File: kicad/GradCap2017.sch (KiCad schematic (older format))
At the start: 14 parts

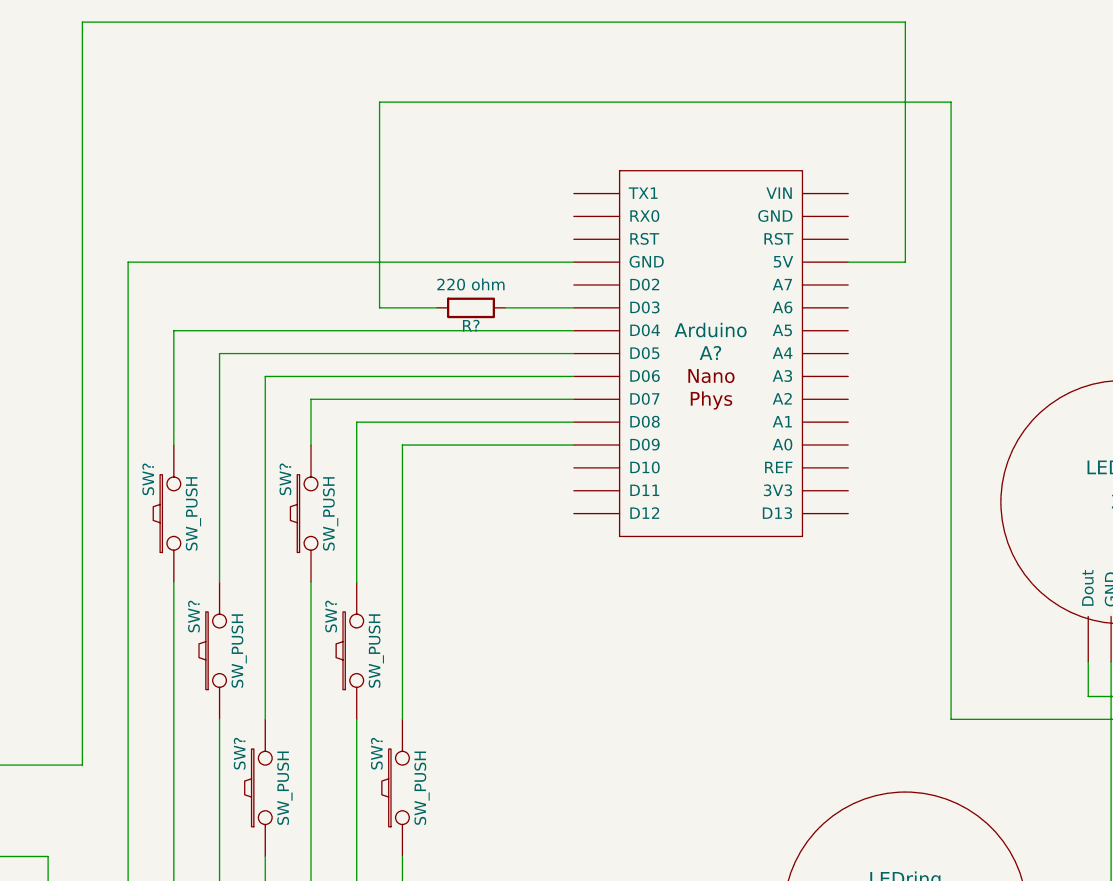
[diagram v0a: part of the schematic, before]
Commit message: add buttons
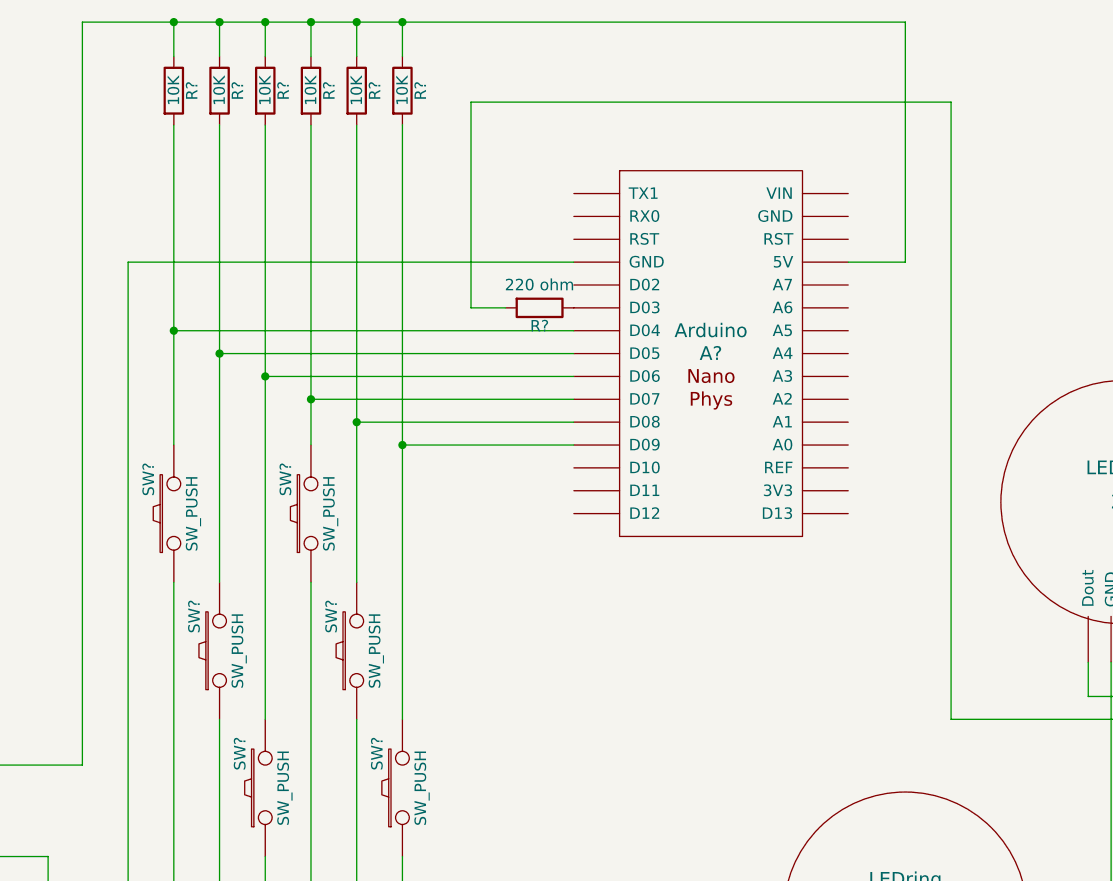
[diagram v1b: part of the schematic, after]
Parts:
- added R? (x6): 10K, symbol R
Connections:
- net at Z?.~ (GND): now also R?.2; no longer Z?.~ (GND)
- net at A?.~ (VIN): now also SW?.2, R?.2; no longer J?.~ (Vout)
- net at A?.~ (VIN), SW?.2: now also R?.2 (x5)
- new net: Z?.~ (GND), Z?.~ (GND)
- new net: A?.~ (VIN), J?.~ (Vout), J?.~ (Vout), SW?.1, SW?.1, SW?.1, SW?.1, SW?.1, SW?.1, Z?.~ (GND), Z?.~ (GND), Z?.~ (GND), Z?.~ (GND)
- new net: J?.~ (Vout), Z?.~ (GND), Z?.~ (GND), Z?.~ (GND), Z?.~ (GND)
- new net: A?.~ (VIN), J?.~ (Vout), R?.1, R?.1, R?.1, R?.1, R?.1, R?.1
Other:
- moved on the sheet: R?
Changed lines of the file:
@@
 L R R?
 U 1 1 5A459198
-P 4900 2200
-F 0 "R?" V 4980 2200 50  0000 C CNN
-F 1 "220 ohm" V 4800 2200 50  0000 C CNN
-F 2 "" V 4830 2200 50  0001 C CNN
-F 3 "" H 4900 2200 50  0001 C CNN
-	1    4900 2200
+P 5200 2200
+F 0 "R?" V 5280 2200 50  0000 C CNN
+F 1 "220 ohm" V 5100 2200 50  0000 C CNN
+F 2 "" V 5130 2200 50  0001 C CNN
+F 3 "" H 5200 2200 50  0001 C CNN
+	1    5200 2200
 	0    1    1    0
 $EndComp
@@
 	3400 2000 5350 2000
 Wire Wire Line
-	5050 2200 5350 2200
-Wire Wire Line
-	4750 2200 4500 2200
-Wire Wire Line
-	4500 2200 4500 1300
-Wire Wire Line
-	4500 1300 7000 1300
+	5050 2200 4900 2200
+Wire Wire Line
+	4900 2200 4900 1300
+Wire Wire Line
+	4900 1300 7000 1300
 Wire Wire Line
 	7000 1300 7000 4000
@@
 	5350 2300 3600 2300
 Wire Wire Line
-	3600 2300 3600 2800
+	3600 1400 3600 2800
 Wire Wire Line
 	5350 2400 3800 2400
 Wire Wire Line
-	3800 2400 3800 3400
+	3800 1400 3800 3400
 Wire Wire Line
 	5350 2500 4000 2500
 Wire Wire Line
-	4000 2500 4000 4000
+	4000 1400 4000 4000
 Wire Wire Line
 	5350 2600 4200 2600
 Wire Wire Line
-	4200 2600 4200 2800
+	4200 1400 4200 2800
 Wire Wire Line
 	5350 2700 4400 2700
 Wire Wire Line
-	4400 2700 4400 3400
+	4400 1400 4400 3400
 Wire Wire Line
 	5350 2800 4600 2800
 Wire Wire Line
-	4600 2800 4600 4000
+	4600 1400 4600 4000
 Wire Wire Line
 	3600 3400 3600 6400
@@
 	4600 4600 4600 6400
 Connection ~ 4600 6400
+$Comp
+L R R?
+U 1 1 5A49671E
+P 3600 1250
+F 0 "R?" V 3680 1250 50  0000 C CNN
+F 1 "10K" V 3600 1250 50  0000 C CNN
+F 2 "" V 3530 1250 30  0000 C CNN
+F 3 "" H 3600 1250 30  0000 C CNN
+	1    3600 1250
+	1    0    0    -1
+$EndComp
+$Comp
+L R R?
+U 1 1 5A496756
+P 3800 1250
+F 0 "R?" V 3880 1250 50  0000 C CNN
+F 1 "10K" V 3800 1250 50  0000 C CNN
+F 2 "" V 3730 1250 30  0000 C CNN
+F 3 "" H 3800 1250 30  0000 C CNN
+	1    3800 1250
+	1    0    0    -1
+$EndComp
+$Comp
+L R R?
+U 1 1 5A496794
+P 4000 1250
+F 0 "R?" V 4080 1250 50  0000 C CNN
+F 1 "10K" V 4000 1250 50  0000 C CNN
+F 2 "" V 3930 1250 30  0000 C CNN
+F 3 "" H 4000 1250 30  0000 C CNN
+	1    4000 1250
+	1    0    0    -1
+$EndComp
+$Comp
+L R R?
+U 1 1 5A4967CE
+P 4200 1250
+F 0 "R?" V 4280 1250 50  0000 C CNN
+F 1 "10K" V 4200 1250 50  0000 C CNN
+F 2 "" V 4130 1250 30  0000 C CNN
+F 3 "" H 4200 1250 30  0000 C CNN
+	1    4200 1250
+	1    0    0    -1
+$EndComp
+$Comp
+L R R?
+U 1 1 5A49680C
+P 4400 1250
+F 0 "R?" V 4480 1250 50  0000 C CNN
+F 1 "10K" V 4400 1250 50  0000 C CNN
+F 2 "" V 4330 1250 30  0000 C CNN
+F 3 "" H 4400 1250 30  0000 C CNN
+	1    4400 1250
+	1    0    0    -1
+$EndComp
+$Comp
+L R R?
+U 1 1 5A4968C0
+P 4600 1250
+F 0 "R?" V 4680 1250 50  0000 C CNN
+F 1 "10K" V 4600 1250 50  0000 C CNN
+F 2 "" V 4530 1250 30  0000 C CNN
+F 3 "" H 4600 1250 30  0000 C CNN
+	1    4600 1250
+	1    0    0    -1
+$EndComp
+Wire Wire Line
+	3600 1100 3600 950
+Connection ~ 3600 950
+Wire Wire Line
+	3800 1100 3800 950
+Connection ~ 3800 950
+Wire Wire Line
+	4000 1100 4000 950
+Connection ~ 4000 950
+Wire Wire Line
+	4200 1100 4200 950
+Connection ~ 4200 950
+Wire Wire Line
+	4400 1100 4400 950
+Connection ~ 4400 950
+Wire Wire Line
+	4600 1100 4600 950
+Connection ~ 4600 950
+Connection ~ 3600 2300
+Connection ~ 3800 2400
+Connection ~ 4000 2500
+Connection ~ 4200 2600
+Connection ~ 4400 2700
+Connection ~ 4600 2800
 $EndSCHEMATC
